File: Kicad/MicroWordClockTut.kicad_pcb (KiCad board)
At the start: 2 copper layers, 20.5 x 20.5 mm, 10 parts, among them J1 USB_B_Micro, J2 Conn_02x03_Male, SW1 SW_SPST_2PIN, U1 ATmega328P-AU, U3 DS1307Z+, U4 8x8_LED_MATRIX, Y1 Crystal

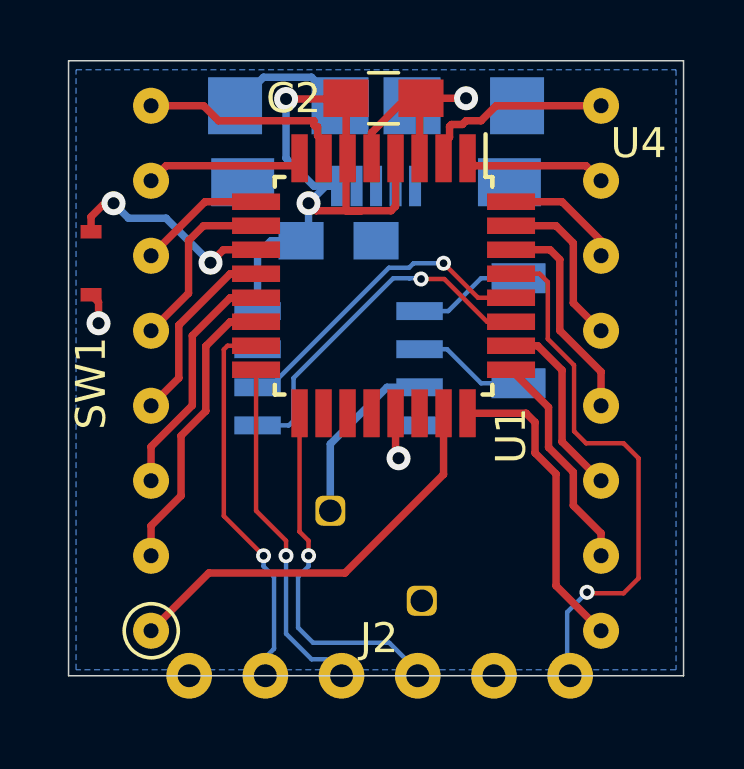
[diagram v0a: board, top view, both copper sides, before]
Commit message: this version released to osh park
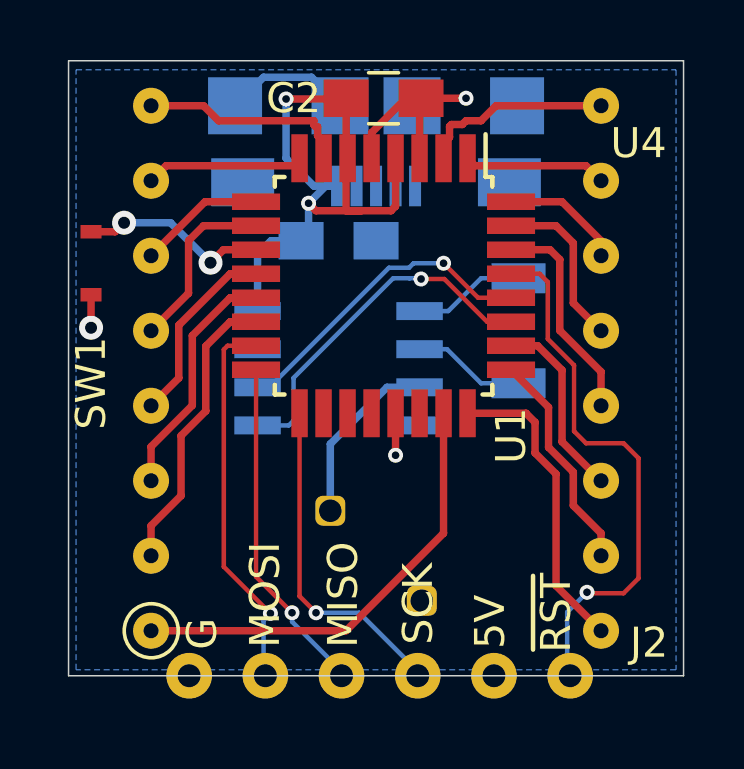
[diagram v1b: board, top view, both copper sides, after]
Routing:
- net /23: track 13.9 -> 15.1 mm
- net /SCK: track 11.4 -> 10.5 mm
- net Net-(SW1-Pad1): track 7.16 -> 6.33 mm
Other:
- board text added: "5V"
- board text added: "G"
- board text added: "MISO"
- board text added: "MOSI"
- board text added: "SCK"
- board text added: "~RST"
